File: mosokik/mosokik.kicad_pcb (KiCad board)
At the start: 2 copper layers, 60 x 60 mm, 54 parts, among them J1 USB2UART, J2 1.47 IPS LCD, J3 ConnBattery, J4 LCD CONN BUFF, J5 TOP_CONN, J7 LCD CONN BUFF, Q1 SS8050, Q2 SS8050, SW1 RST, SW3 Boot, U1 CH340C, U2 ESP32-S3-WROOM-1, U4 TPS63001_SEPIC_3V3, U5 BQ24075RGT_DPPM, U7 MAX17048G+T10

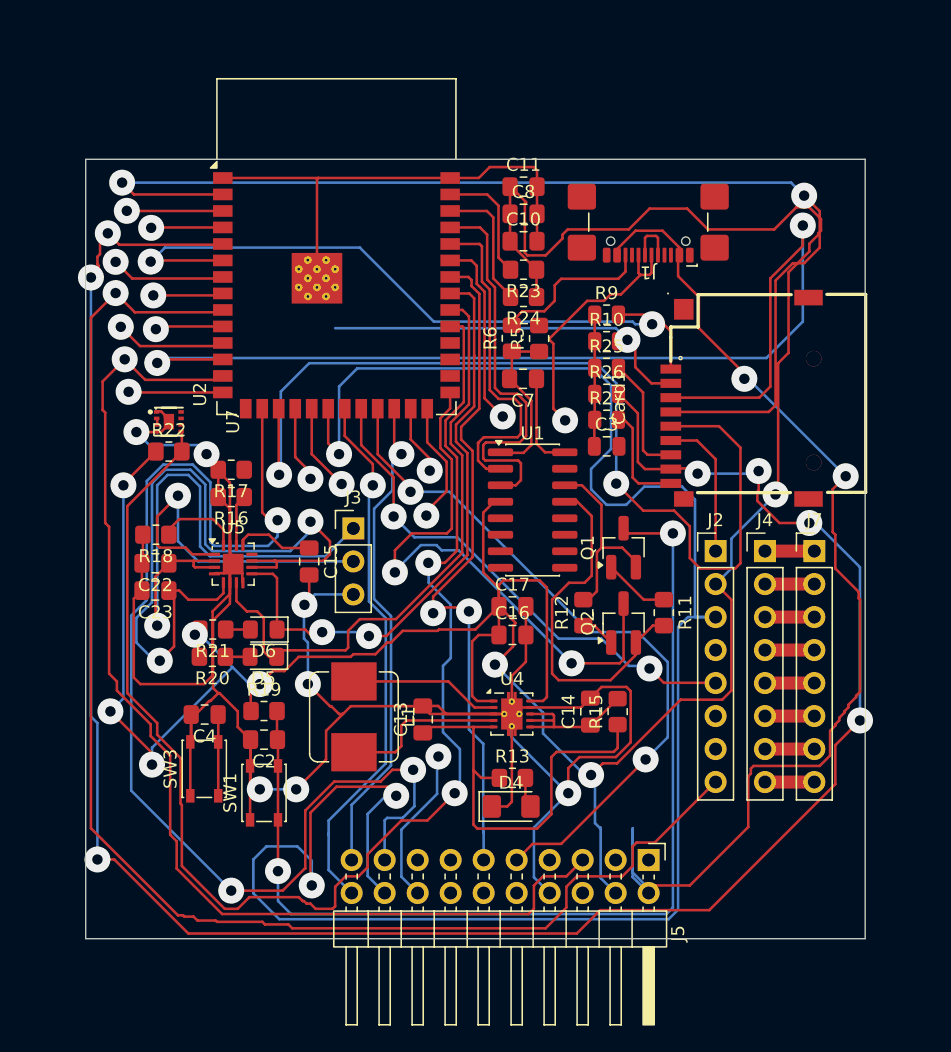
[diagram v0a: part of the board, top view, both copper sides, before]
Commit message: unrouted 8 pieces
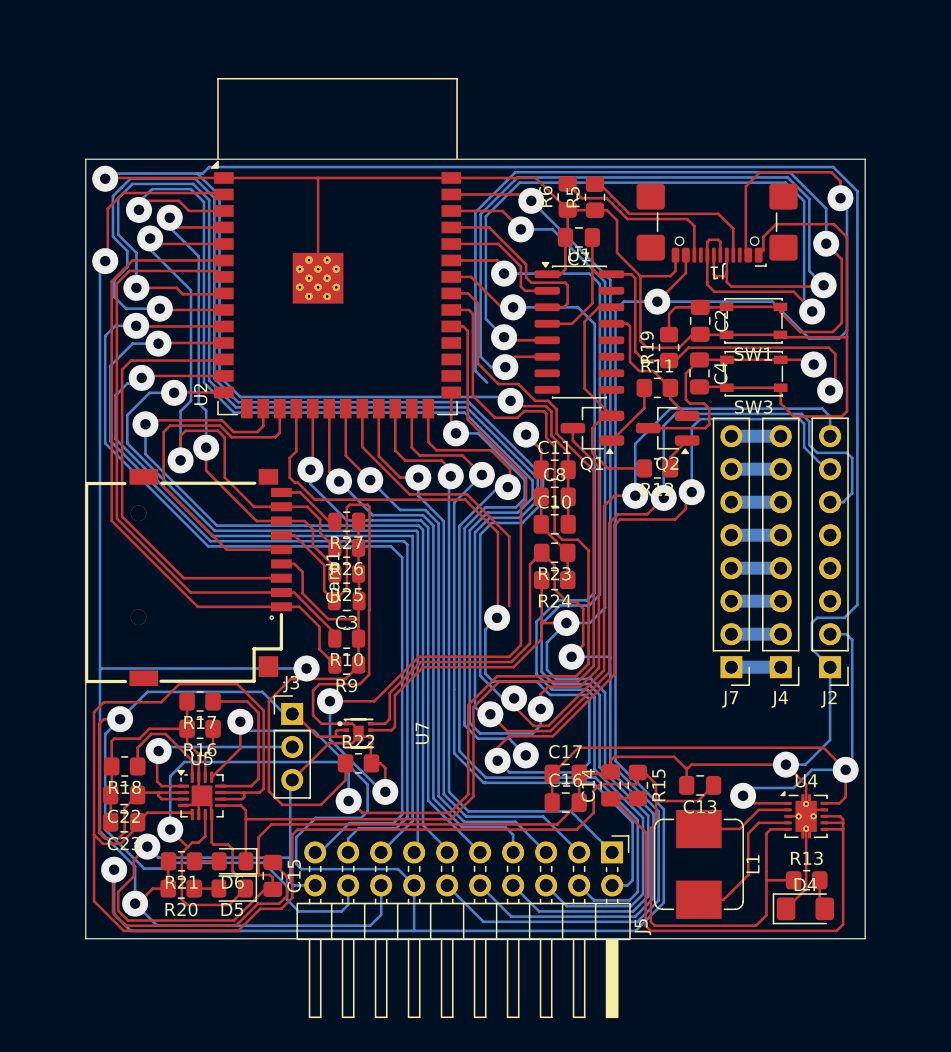
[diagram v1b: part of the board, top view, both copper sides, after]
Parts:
- moved SW1 52.3 mm to (171.1, 81.2), turned to 180 degrees
- moved SW3 52.1 mm to (171.1, 85.3), turned to 180 degrees
- moved C2 46.5 mm to (167.0, 81.2), turned to -90 degrees
- moved C4 46.3 mm to (166.9, 85.3), turned to -90 degrees
- moved Card1 42.9 mm to (129.5, 101.0), turned to -90 degrees
- moved R19 41.9 mm to (164.6, 83.3), turned to 90 degrees
- moved R9 33.6 mm to (139.8, 107.7), turned to 180 degrees
- moved R10 30.4 mm to (139.8, 105.7), turned to 180 degrees
- moved L1 28.9 mm to (166.9, 123.1)
- moved R22 28.1 mm to (140.7, 115.3)
- moved U7 28.1 mm to (140.7, 113.0)
- moved R25 25.5 mm to (139.8, 100.7), turned to 180 degrees
- moved C15 24.4 mm to (134.1, 124.0)
- moved D4 24.0 mm to (175.1, 126.5)
- moved R13 24.0 mm to (175.2, 124.3)
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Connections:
- J5 pad 1: /IO17 -> /IO47
- J5 pad 10: /IO48 -> /SCL
- J5 pad 11: /IO41 -> /IO46
- J5 pad 13: /IO42 -> /IO20
- J5 pad 14: /SCL -> VBUS
- J5 pad 15: /IO45 -> /IO19
- J5 pad 16: /MOSI -> +3.3V
- J5 pad 17: /IO46 -> /IO18
- J5 pad 18: /SCK -> +BATT
- J5 pad 19: /IO47 -> /IO17
- J5 pad 2: VBUS -> /IO48
- J5 pad 20: /MISO -> GND
- J5 pad 3: /IO18 -> /IO21
- J5 pad 4: +3.3V -> /IO45
- J5 pad 5: /IO19 -> /MISO
- J5 pad 6: +BATT -> /IO41
- J5 pad 7: /IO20 -> /SCK
- J5 pad 8: GND -> /IO42
- J5 pad 9: /IO21 -> /MOSI
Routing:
- net GND: track 260.2 -> 469.6 mm, vias 7 -> 4
- net /DC: track 5.41 -> 142.8 mm, vias 1 -> 3
- net /DAT1: track 167.5 -> 44.6 mm, vias 7 -> 2
- net VBUS: track 91.6 -> 205.9 mm, vias 2 -> 4
- net /SDA: track 9.39 -> 118.9 mm, vias 0 -> 2
- net /SCK: track 152.1 -> 44.2 mm, vias 3 -> 1
- net /CS: track 6.34 -> 105.9 mm, vias 1 -> 3
- net /SCL: track 10.2 -> 108.3 mm, vias 0 -> 2
- net /EN: track 86.0 -> 179.7 mm
- net +3.3V: track 332.3 -> 257.8 mm, vias 10 -> 7
- net /IO17: track 4.94 -> 71.9 mm
- net /IO42: track 14.6 -> 79.5 mm
- net /IO18: track 8.56 -> 68.7 mm
- net Net-(U1-UD-): track 3.78 -> 63.6 mm, vias 0 -> 2
- net /IO20: track 7.34 -> 60.3 mm
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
